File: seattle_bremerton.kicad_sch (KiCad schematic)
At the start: 20 parts

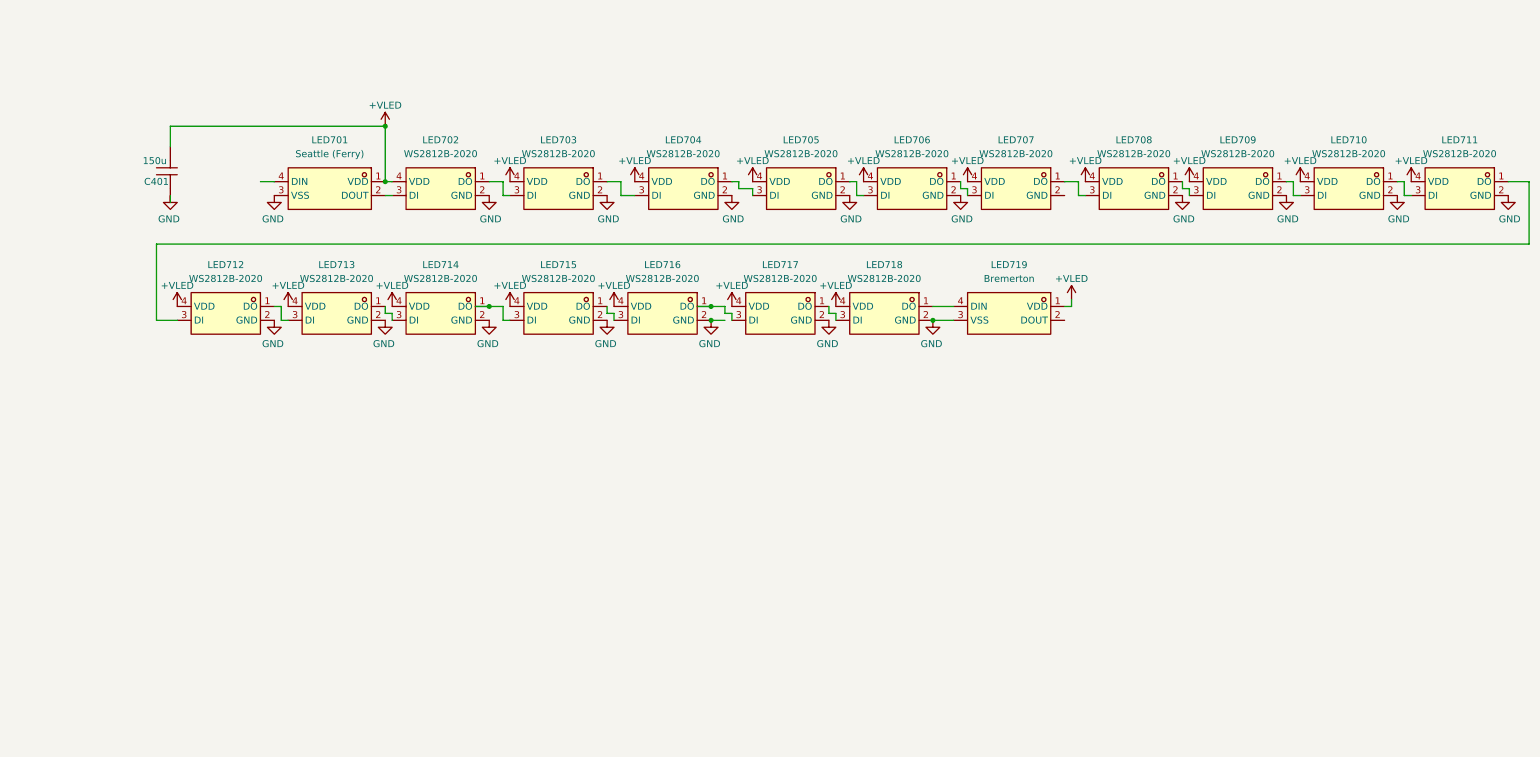
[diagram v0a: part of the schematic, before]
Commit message: junction checkpoint
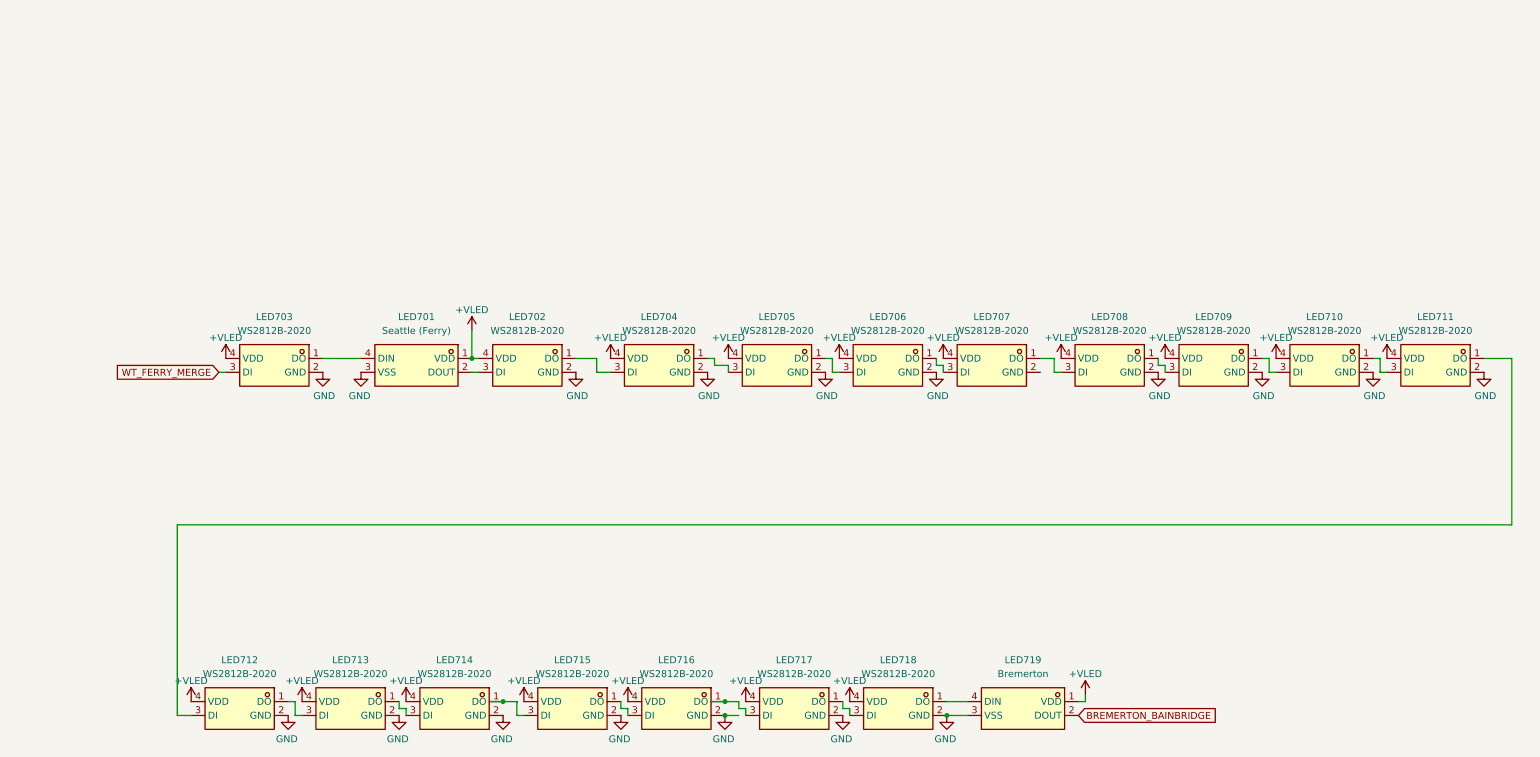
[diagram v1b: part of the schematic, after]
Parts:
- removed C401: 150u, EasyEDA:CAP-SMD_L3.5-W2.8, symbol EasyEDA:CL21B106KOQNNNE
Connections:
- net at LED703.1 (DO): now also LED701.4 (DIN); no longer LED704.3 (DI)
- net at LED702.1 (DO): now also LED704.3 (DI); no longer LED703.3 (DI)
- net BREMERTON_BAINBRIDGE: now reaches LED719.2 (DOUT)
- new net WT_FERRY_MERGE: LED703.3 (DI)
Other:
- moved on the sheet: LED701, LED702, LED704, LED705, LED706, LED707, LED708, LED709, LED710, LED711, LED712, LED713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
